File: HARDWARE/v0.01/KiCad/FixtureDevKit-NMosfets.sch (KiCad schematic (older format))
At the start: 32 parts, among them J71 NFET_0, J72 NFET_4, J73 NFET_1, J74 NFET_5, J75 NFET_2, J76 NFET_6, J77 NFET_3, J78 NFET_7, Q13 FDN337N, Q14 FDN337N, Q15 FDN337N, Q16 FDN337N, Q17 FDN337N, Q18 FDN337N, Q19 FDN337N, Q20 FDN337N

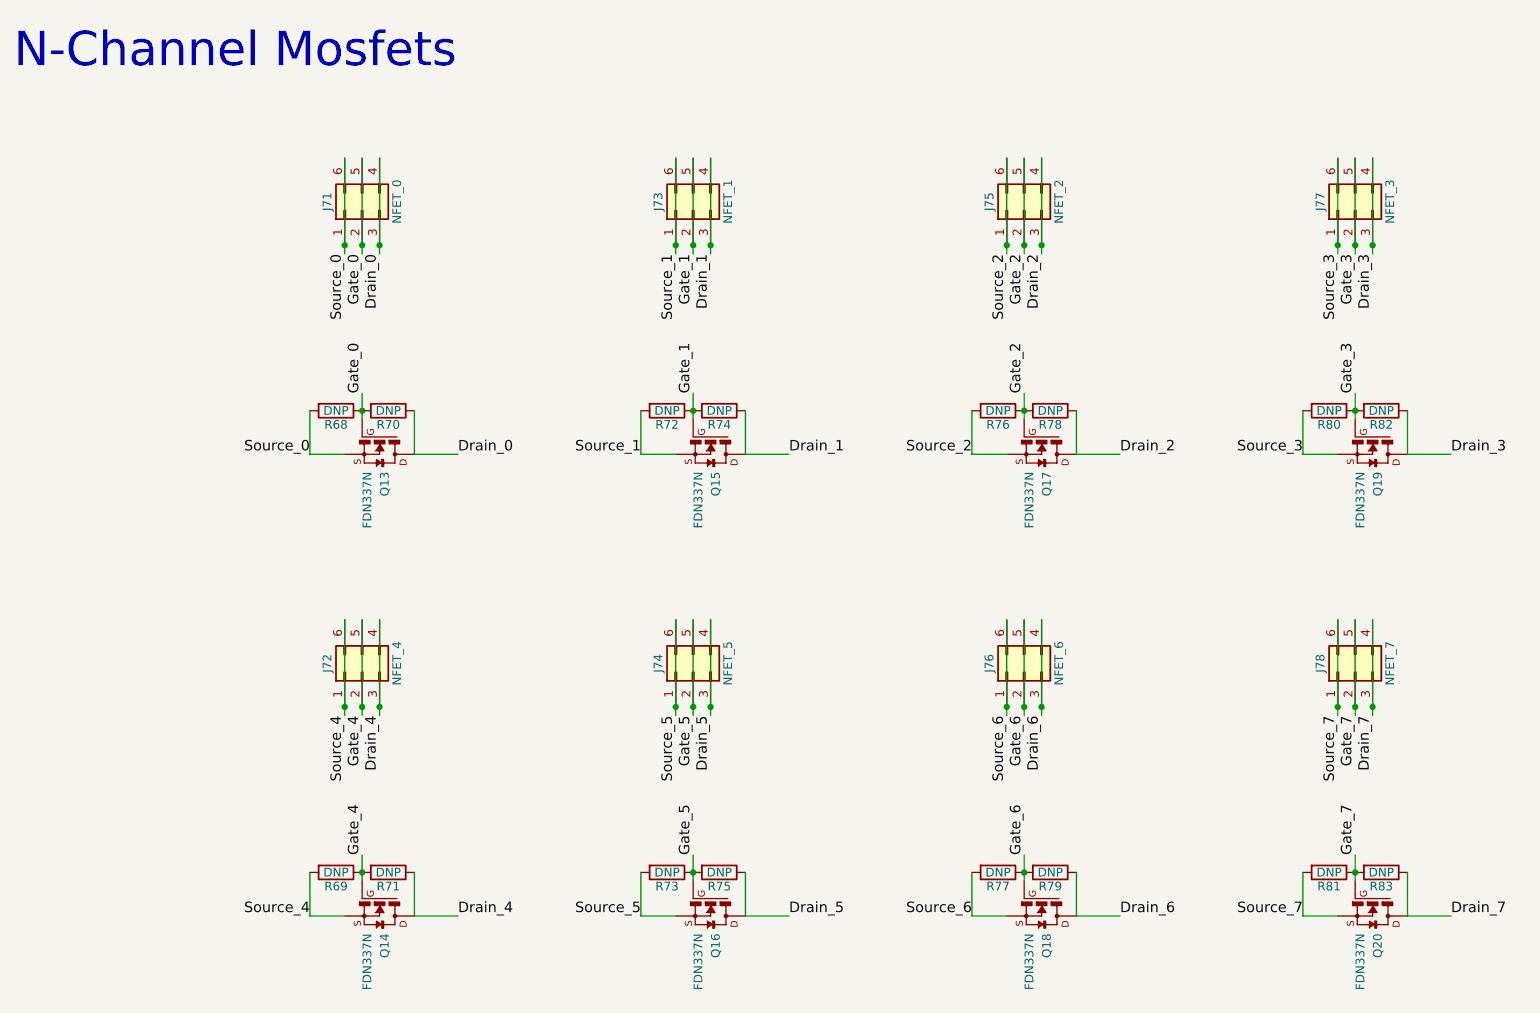
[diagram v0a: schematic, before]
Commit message: updating pcb layout
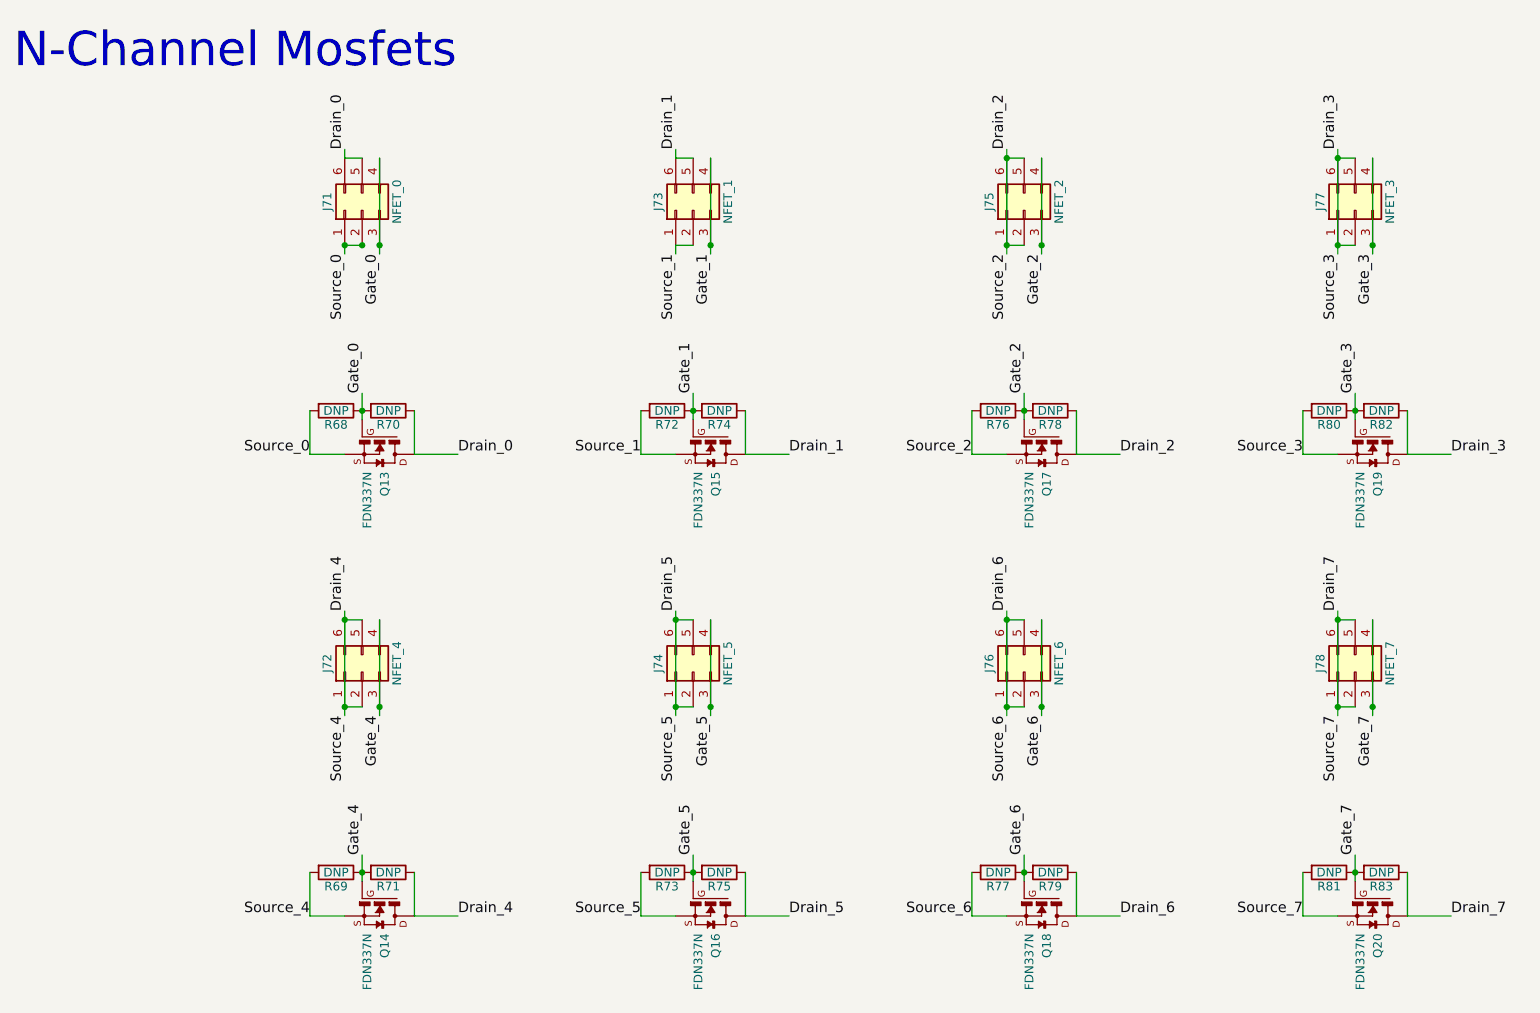
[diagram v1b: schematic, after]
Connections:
- net Source_2 is gone; now on net Drain_2: J75.1 (Pin_1), J75.6 (Pin_6), Q17.2 (S), R76.2
- net Source_3 is gone; now on net Drain_3: J77.1 (Pin_1), J77.6 (Pin_6), Q19.2 (S), R80.2
- net Source_4 is gone; now on net Drain_4: J72.1 (Pin_1), J72.6 (Pin_6), Q14.2 (S), R69.2
- net Source_5 is gone; now on net Drain_5: J74.1 (Pin_1), J74.6 (Pin_6), Q16.2 (S), R73.2
- net Source_6 is gone; now on net Drain_6: J76.1 (Pin_1), J76.6 (Pin_6), Q18.2 (S), R77.2
- net Source_7 is gone; now on net Drain_7: J78.1 (Pin_1), J78.6 (Pin_6), Q20.2 (S), R81.2
- net Drain_0: now also J71.5 (Pin_5), J71.6 (Pin_6); no longer J71.3 (Pin_3), J71.4 (Pin_4)
- net Drain_1: now also J73.5 (Pin_5), J73.6 (Pin_6); no longer J73.3 (Pin_3), J73.4 (Pin_4)
- net Drain_2: now also J75.2 (Pin_2), J75.5 (Pin_5); no longer J75.3 (Pin_3), J75.4 (Pin_4)
- net Drain_3: now also J77.2 (Pin_2), J77.5 (Pin_5); no longer J77.3 (Pin_3), J77.4 (Pin_4)
- net Drain_4: now also J72.2 (Pin_2), J72.5 (Pin_5); no longer J72.3 (Pin_3), J72.4 (Pin_4)
- net Drain_5: now also J74.2 (Pin_2), J74.5 (Pin_5); no longer J74.3 (Pin_3), J74.4 (Pin_4)
- net Drain_6: now also J76.2 (Pin_2), J76.5 (Pin_5); no longer J76.3 (Pin_3), J76.4 (Pin_4)
- net Drain_7: now also J78.2 (Pin_2), J78.5 (Pin_5); no longer J78.3 (Pin_3), J78.4 (Pin_4)
- net Gate_0: now also J71.3 (Pin_3), J71.4 (Pin_4); no longer J71.2 (Pin_2), J71.5 (Pin_5)
- net Gate_1: now also J73.3 (Pin_3), J73.4 (Pin_4); no longer J73.2 (Pin_2), J73.5 (Pin_5)
- net Gate_2: now also J75.3 (Pin_3), J75.4 (Pin_4); no longer J75.2 (Pin_2), J75.5 (Pin_5)
- net Gate_3: now also J77.3 (Pin_3), J77.4 (Pin_4); no longer J77.2 (Pin_2), J77.5 (Pin_5)
- net Gate_4: now also J72.3 (Pin_3), J72.4 (Pin_4); no longer J72.2 (Pin_2), J72.5 (Pin_5)
- net Gate_5: now also J74.3 (Pin_3), J74.4 (Pin_4); no longer J74.2 (Pin_2), J74.5 (Pin_5)
- net Gate_6: now also J76.3 (Pin_3), J76.4 (Pin_4); no longer J76.2 (Pin_2), J76.5 (Pin_5)
- net Gate_7: now also J78.3 (Pin_3), J78.4 (Pin_4); no longer J78.2 (Pin_2), J78.5 (Pin_5)
- net Source_0: now also J71.2 (Pin_2); no longer J71.6 (Pin_6)
- net Source_1: now also J73.2 (Pin_2); no longer J73.6 (Pin_6)
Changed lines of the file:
@@
 Text Label 2400 1800 3    60   ~ 0
 Source_0
-Text Label 2500 1800 3    60   ~ 0
+Text Label 2600 1800 3    60   ~ 0
 Gate_0
-Text Label 2600 1800 3    60   ~ 0
+Text Label 2400 1200 1    60   ~ 0
 Drain_0
 Text Label 2500 2600 1    60   ~ 0
@@
 Wire Wire Line
 	2200 2950 2400 2950
-Wire Wire Line
-	2600 1250 2600 1800
-Wire Wire Line
-	2500 1250 2500 1800
-Wire Wire Line
-	2400 1250 2400 1800
 Connection ~ 2400 1750
 Connection ~ 2500 1750
@@
 Wire Wire Line
 	2800 5600 3050 5600
-Connection ~ 2600 4400
-Connection ~ 2500 4400
 Connection ~ 2400 4400
 Wire Wire Line
-	2400 3900 2400 4450
-Wire Wire Line
-	2500 3900 2500 4450
-Wire Wire Line
-	2600 3900 2600 4450
+	2400 3850 2400 4450
 Wire Wire Line
 	2200 5600 2400 5600
@@
 Text Label 2500 5250 1    60   ~ 0
 Gate_4
+Text Label 2400 3850 1    60   ~ 0
+Drain_4
 Text Label 2600 4450 3    60   ~ 0
-Drain_4
-Text Label 2500 4450 3    60   ~ 0
 Gate_4
 Text Label 2400 4450 3    60   ~ 0
@@
 Wire Wire Line
 	4700 5600 4950 5600
-Connection ~ 8300 4400
-Connection ~ 8200 4400
 Connection ~ 8100 4400
 Wire Wire Line
-	8100 3900 8100 4450
-Wire Wire Line
-	8200 3900 8200 4450
-Wire Wire Line
-	8300 3900 8300 4450
+	8100 3850 8100 4450
 Wire Wire Line
 	7900 5600 8100 5600
@@
 Text Label 8200 5250 1    60   ~ 0
 Gate_7
+Text Label 8100 3850 1    60   ~ 0
+Drain_7
 Text Label 8300 4450 3    60   ~ 0
-Drain_7
-Text Label 8200 4450 3    60   ~ 0
 Gate_7
 Text Label 8100 4450 3    60   ~ 0
@@
 	0    1    1    0
 $EndComp
-Connection ~ 6400 4400
-Connection ~ 6300 4400
 Connection ~ 6200 4400
 Wire Wire Line
-	6200 3900 6200 4450
-Wire Wire Line
-	6300 3900 6300 4450
-Wire Wire Line
-	6400 3900 6400 4450
+	6200 3850 6200 4450
 Wire Wire Line
 	6000 5600 6200 5600
@@
 Text Label 6300 5250 1    60   ~ 0
 Gate_6
+Text Label 6200 3850 1    60   ~ 0
+Drain_6
 Text Label 6400 4450 3    60   ~ 0
-Drain_6
-Text Label 6300 4450 3    60   ~ 0
 Gate_6
 Text Label 6200 4450 3    60   ~ 0
@@
 	0    1    1    0
 $EndComp
-Connection ~ 4500 4400
-Connection ~ 4400 4400
 Connection ~ 4300 4400
 Wire Wire Line
-	4300 3900 4300 4450
-Wire Wire Line
-	4400 3900 4400 4450
-Wire Wire Line
-	4500 3900 4500 4450
+	4300 3850 4300 4450
 Wire Wire Line
 	4100 5600 4300 5600
@@
 Text Label 4400 5250 1    60   ~ 0
 Gate_5
+Text Label 4300 3850 1    60   ~ 0
+Drain_5
 Text Label 4500 4450 3    60   ~ 0
-Drain_5
-Text Label 4400 4450 3    60   ~ 0
 Gate_5
 Text Label 4300 4450 3    60   ~ 0
@@
 Wire Wire Line
 	4700 2950 4950 2950
-Connection ~ 8300 1750
-Connection ~ 8200 1750
 Connection ~ 8100 1750
 Wire Wire Line
-	8100 1250 8100 1800
-Wire Wire Line
-	8200 1250 8200 1800
-Wire Wire Line
-	8300 1250 8300 1800
+	8100 1200 8100 1800
 Wire Wire Line
 	7900 2950 8100 2950
@@
 Text Label 8200 2600 1    60   ~ 0
 Gate_3
+Text Label 8100 1200 1    60   ~ 0
+Drain_3
 Text Label 8300 1800 3    60   ~ 0
-Drain_3
-Text Label 8200 1800 3    60   ~ 0
 Gate_3
 Text Label 8100 1800 3    60   ~ 0
@@
 	0    1    1    0
 $EndComp
-Connection ~ 6400 1750
-Connection ~ 6300 1750
 Connection ~ 6200 1750
 Wire Wire Line
-	6200 1250 6200 1800
-Wire Wire Line
-	6300 1250 6300 1800
-Wire Wire Line
-	6400 1250 6400 1800
+	6200 1200 6200 1800
 Wire Wire Line
 	6000 2950 6200 2950
@@
 Text Label 6300 2600 1    60   ~ 0
 Gate_2
+Text Label 6200 1200 1    60   ~ 0
+Drain_2
 Text Label 6400 1800 3    60   ~ 0
-Drain_2
-Text Label 6300 1800 3    60   ~ 0
 Gate_2
 Text Label 6200 1800 3    60   ~ 0
@@
 	0    1    1    0
 $EndComp
-Connection ~ 4500 1750
-Connection ~ 4400 1750
-Connection ~ 4300 1750
-Wire Wire Line
-	4300 1250 4300 1800
-Wire Wire Line
-	4400 1250 4400 1800
-Wire Wire Line
-	4500 1250 4500 1800
 Wire Wire Line
 	4100 2950 4300 2950
@@
 Text Label 4400 2600 1    60   ~ 0
 Gate_1
+Text Label 4300 1200 1    60   ~ 0
+Drain_1
 Text Label 4500 1800 3    60   ~ 0
-Drain_1
-Text Label 4400 1800 3    60   ~ 0
 Gate_1
 Text Label 4300 1800 3    60   ~ 0
@@
 	0    1    1    0
 $EndComp
+Wire Wire Line
+	2500 1750 2400 1750
+Wire Wire Line
+	2400 1750 2400 1800
+Wire Wire Line
+	2600 1250 2600 1800
+Wire Wire Line
+	2500 1250 2400 1250
+Wire Wire Line
+	2400 1250 2400 1200
+Wire Wire Line
+	4300 1800 4300 1750
+Wire Wire Line
+	4300 1750 4400 1750
+Wire Wire Line
+	4500 1250 4500 1800
+Connection ~ 4500 1750
+Wire Wire Line
+	4400 1250 4300 1250
+Wire Wire Line
+	4300 1250 4300 1200
+Wire Wire Line
+	6200 1750 6300 1750
+Wire Wire Line
+	6400 1250 6400 1800
+Connection ~ 6400 1750
+Wire Wire Line
+	6300 1250 6200 1250
+Connection ~ 6200 1250
+Wire Wire Line
+	8100 1750 8200 1750
+Wire Wire Line
+	8300 1250 8300 1800
+Connection ~ 8300 1750
+Wire Wire Line
+	8200 1250 8100 1250
+Connection ~ 8100 1250
+Wire Wire Line
+	2400 4400 2500 4400
+Wire Wire Line
+	2600 3900 2600 4450
+Connection ~ 2600 4400
+Wire Wire Line
+	2500 3900 2400 3900
+Connection ~ 2400 3900
+Wire Wire Line
+	4300 4400 4400 4400
+Wire Wire Line
+	4500 3900 4500 4450
+Connection ~ 4500 4400
+Wire Wire Line
+	4400 3900 4300 3900
+Connection ~ 4300 3900
+Wire Wire Line
+	6200 4400 6300 4400
+Wire Wire Line
+	6400 3900 6400 4450
+Connection ~ 6400 4400
+Wire Wire Line
+	6300 3900 6200 3900
+Connection ~ 6200 3900
+Wire Wire Line
+	8100 4400 8200 4400
+Wire Wire Line
+	8300 3900 8300 4450
+Connection ~ 8300 4400
+Wire Wire Line
+	8200 3900 8100 3900
+Connection ~ 8100 3900
 $EndSCHEMATC
